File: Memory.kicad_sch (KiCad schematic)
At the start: 8 parts, among them U3 28C256, U4 74HC32, U5 62256, U6 74HC32, U7 74HC00, U8 62256, U9 74HC04

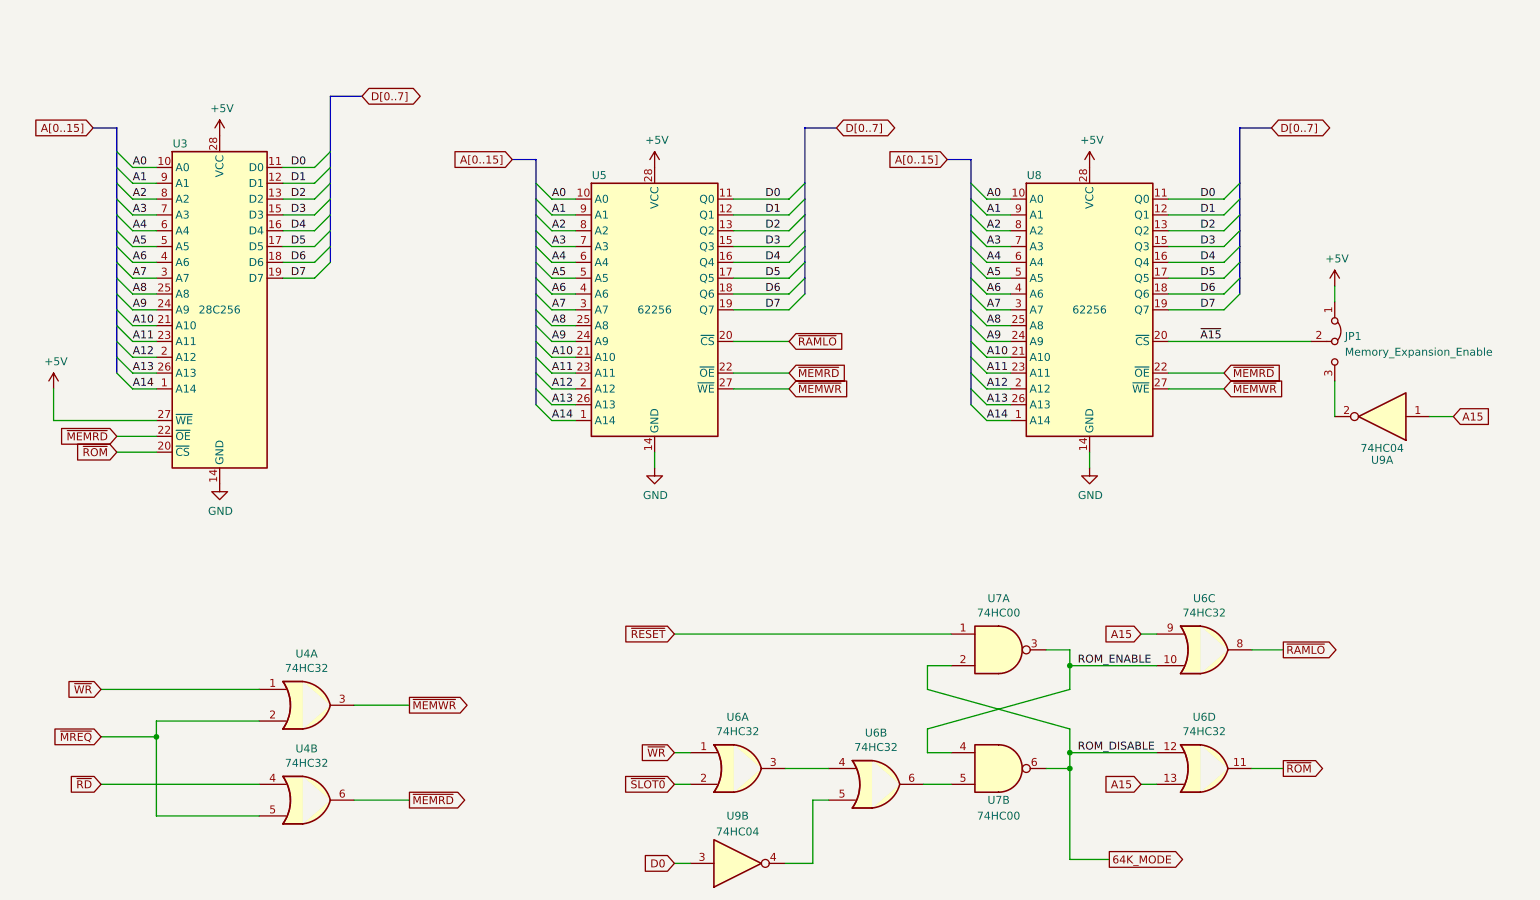
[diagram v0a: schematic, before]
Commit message: Schematic cleanup
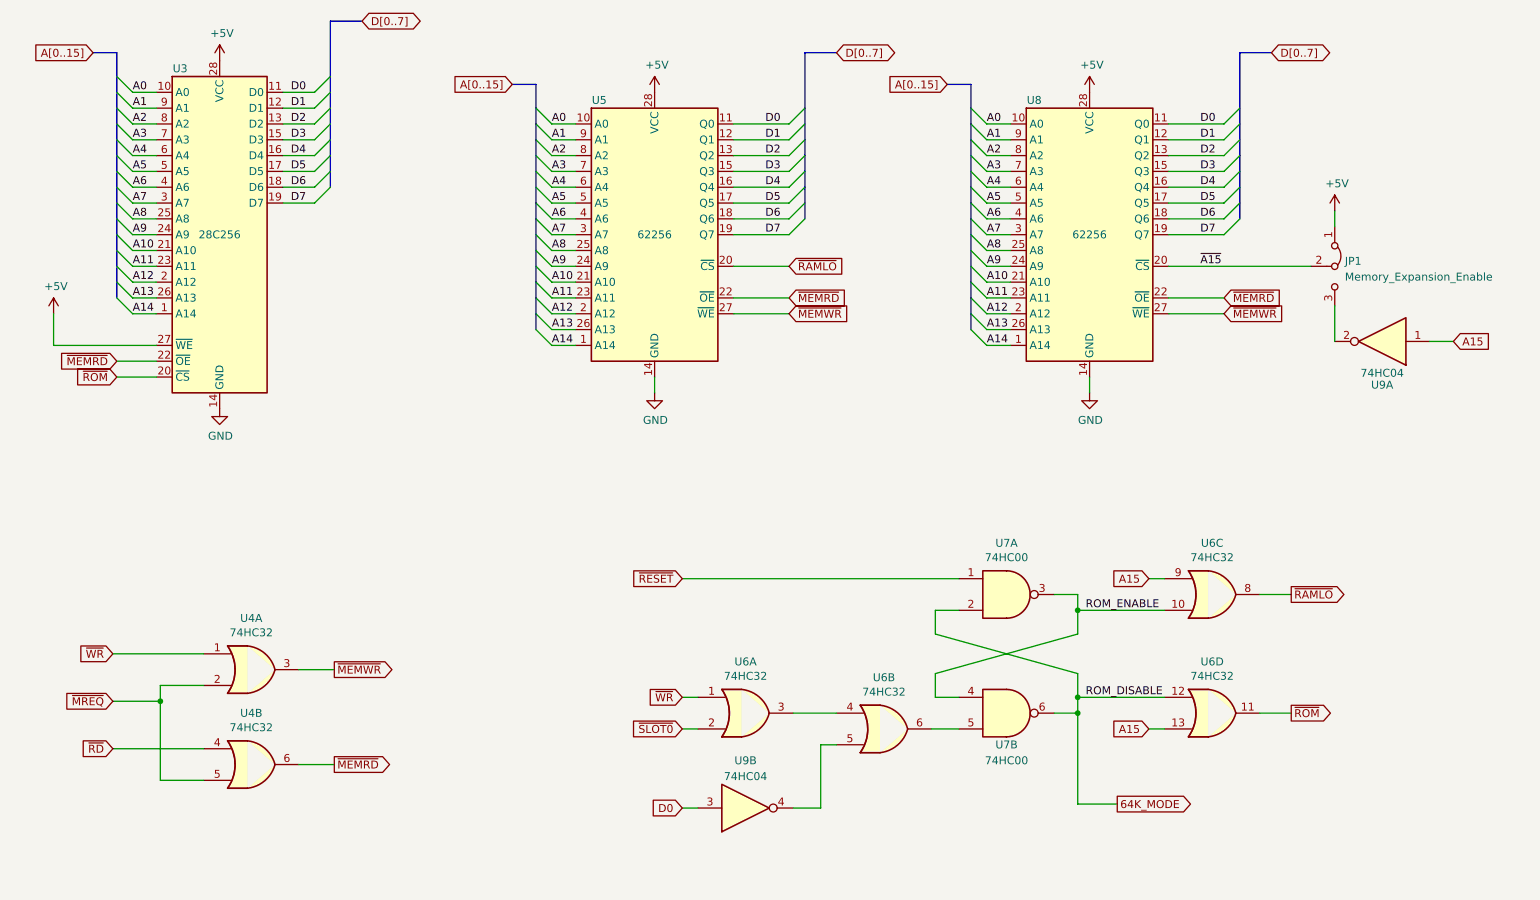
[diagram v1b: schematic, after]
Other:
- moved on the sheet: JP1, U3, U4A, U4B, U5, U6A, U6B, U6C, U6D, U7A, U7B, U8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
